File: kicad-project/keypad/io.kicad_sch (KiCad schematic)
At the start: 18 parts, among them SW1 RotaryEncoder, SW2 RotaryEncoder, SW25 SW_RST

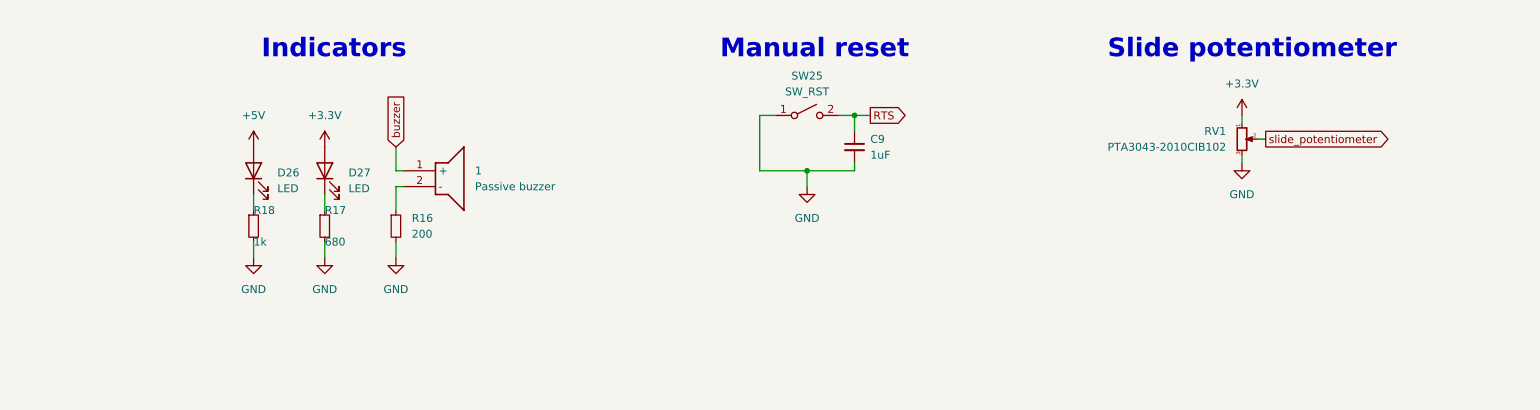
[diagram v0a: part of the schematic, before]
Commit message: correct schematic
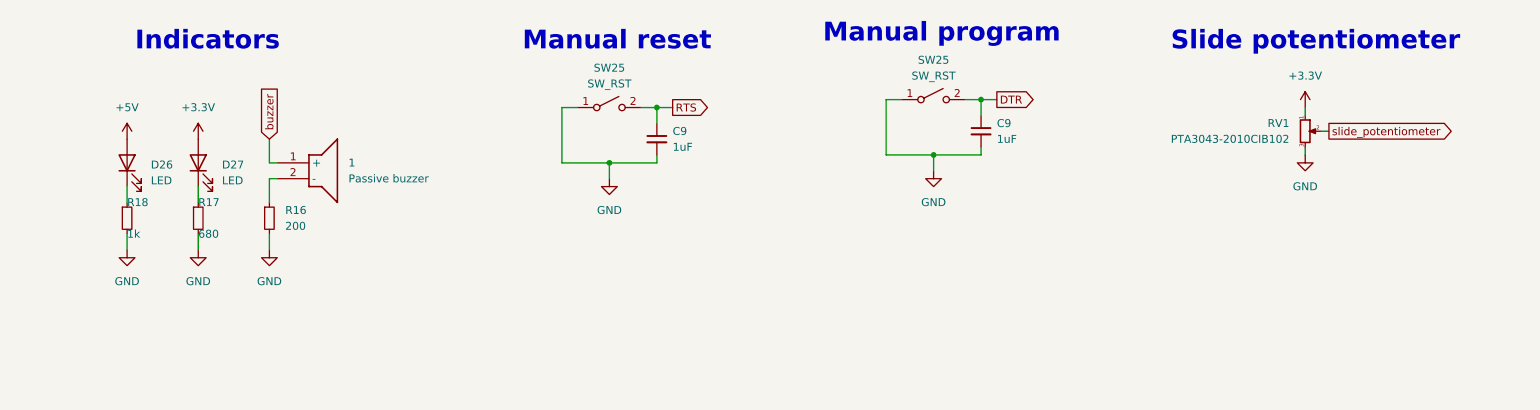
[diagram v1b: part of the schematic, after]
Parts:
- added C9: 1uF, Capacitor_SMD:C_0603_1608Metric, symbol PutRocketLab_RCL:C_Small
- added SW25: SW_RST, Button_Switch_THT:SW_PUSH_6mm, symbol Switch:SW_SPST
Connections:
- net GND: now also C9.2, SW25.1 (A)
- new net DTR: C9.1, SW25.2 (B)
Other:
- note added: "Manual program"
- moved on the sheet: 1, C9, D26, D27, R16, R17, R18, RV1, SW25
